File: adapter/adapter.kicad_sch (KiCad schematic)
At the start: 11 parts, among them J1 Serial, J2 Conn_01x05_Female, J3 Conn_01x06_Female, J4 RGB, J7 Trackball, SW1 Reset, U1 STM32F401 / STM32F411 Blackpi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

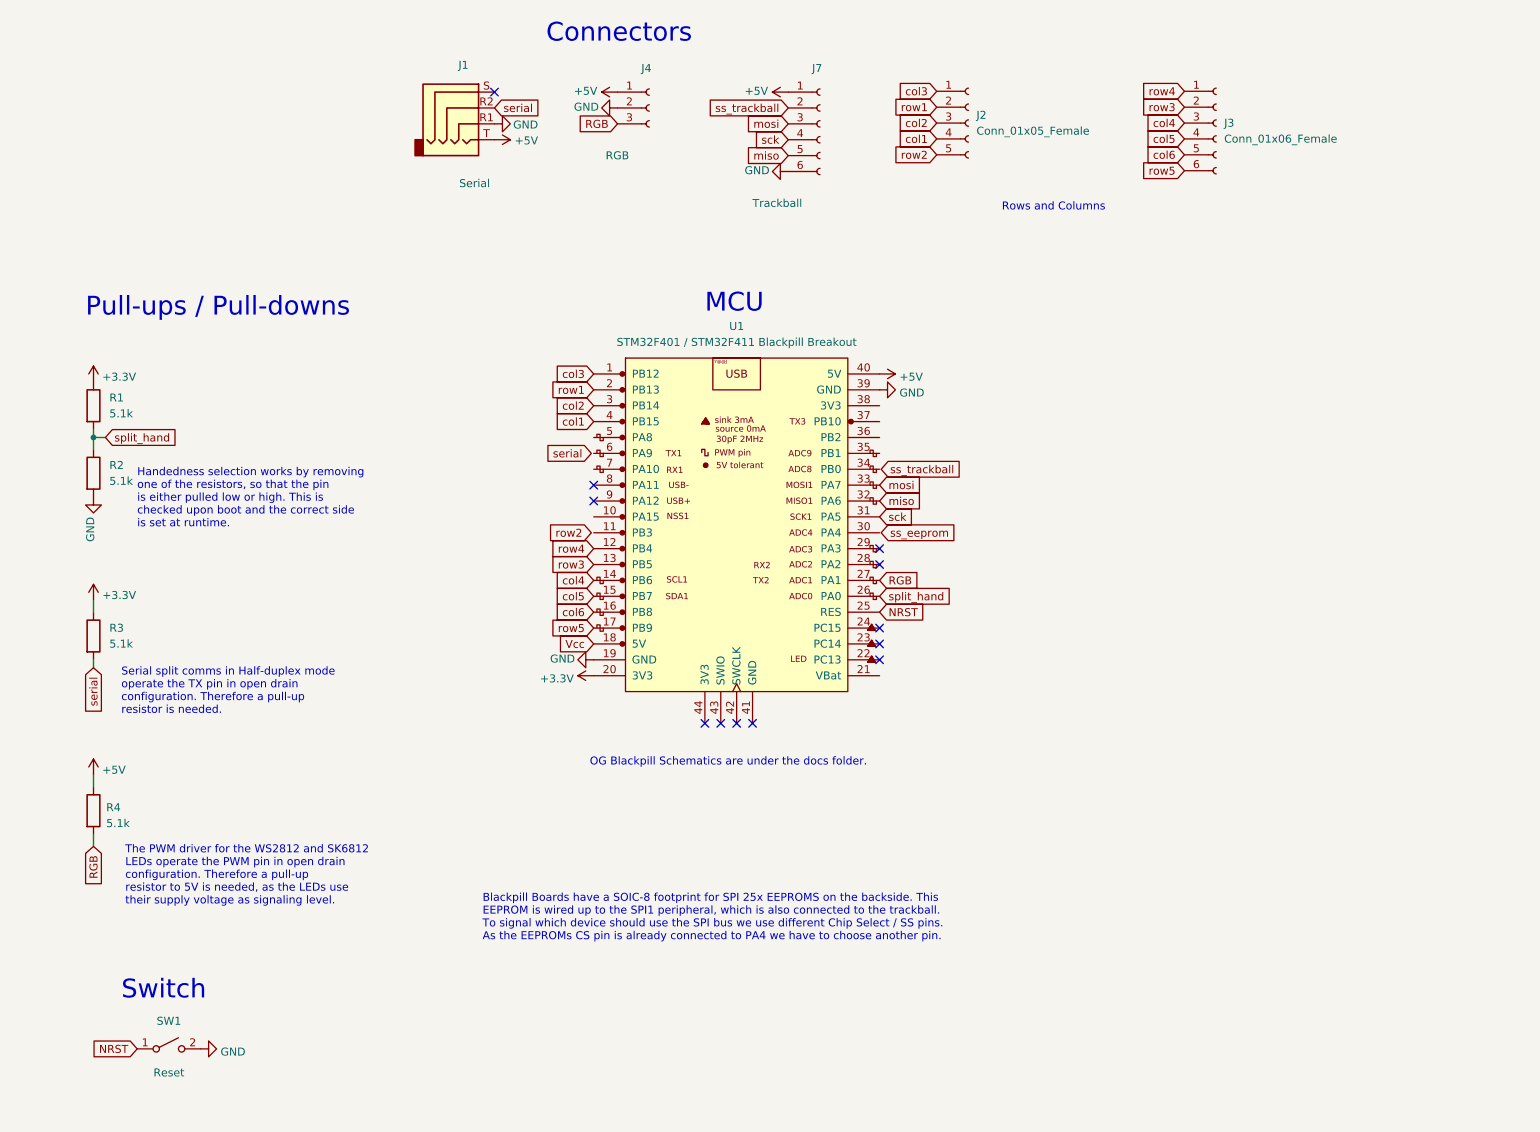
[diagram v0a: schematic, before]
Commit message: Update schematic for left and right hand
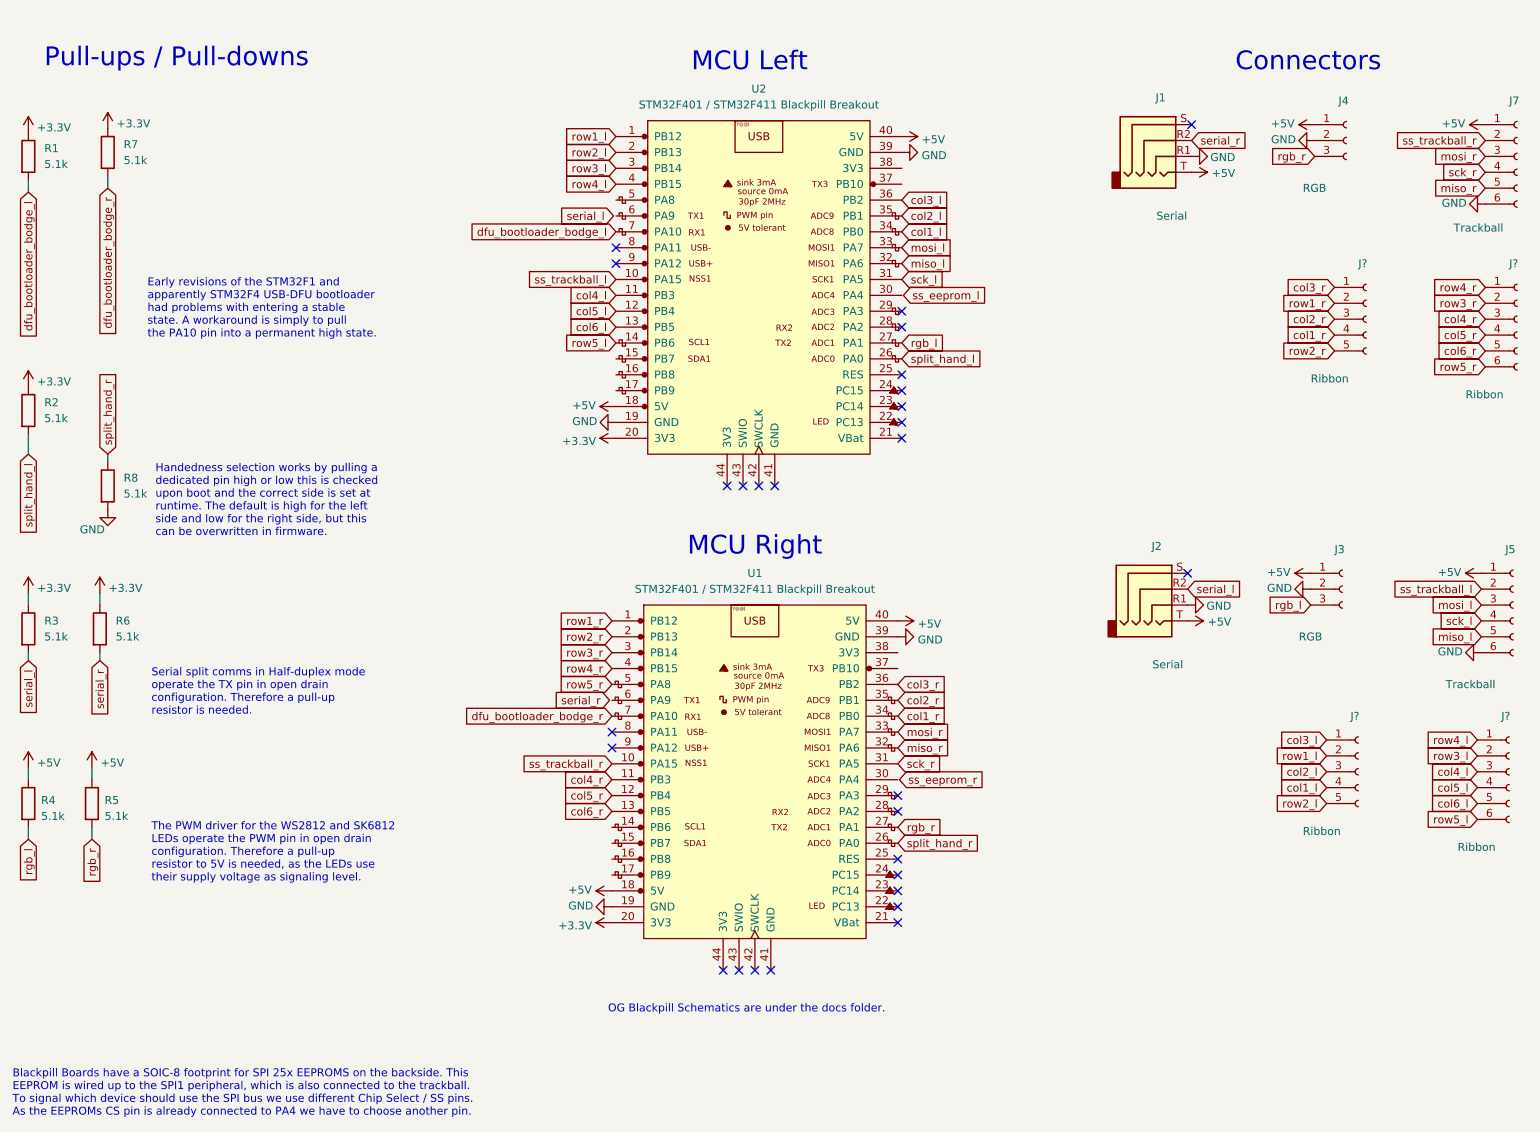
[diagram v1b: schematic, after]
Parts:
- removed J2: Conn_01x05_Female, customs:PinHeader_1x05_P2.54mm_Vertical, symbol Connector:Conn_01x05_Female
- removed J3: Conn_01x06_Female, Connector_PinHeader_2.54mm:PinHeader_1x06_P2.54mm_Vertical, symbol Connector:Conn_01x06_Female
- removed SW1: Reset, customs:switch_rst, symbol Switch:SW_SPST
- added J2: Serial, Library:Jack_3.5mm_PJ320E_Horizontal, symbol Connector:AudioJack4
- added J3: RGB, Connector_PinSocket_2.54mm:PinSocket_1x03_P2.54mm_Vertical, symbol Connector:Conn_01x03_Female
- added J5: Trackball, Connector_PinHeader_2.54mm:PinHeader_1x06_P2.54mm_Vertical, symbol Connector:Conn_01x06_Female
- added J? (x2): Ribbon, customs:PinHeader_1x05_P2.54mm_Vertical, symbol Connector:Conn_01x05_Female
- added J? (x2): Ribbon, Connector_PinHeader_2.54mm:PinHeader_1x06_P2.54mm_Vertical, symbol Connector:Conn_01x06_Female
- added R1, R5, R6, R7: 5.1k, Resistor_SMD:R_0805_2012Metric_Pad1.20x1.40mm_HandSolder, symbol Device:R
- added U1: STM32F401 / STM32F411 Blackpill Breakout, Library:YAAJ_WeAct_BlackPill_SWD_2, symbol YAAJ_WeAct_BlackPill_Part_Like_SWD_Breakout:YAAJ_WeAct_BlackPill_Part_Like_SWD_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
- J1, J4, J7: JLCPCB BOM (none) -> 0
- R2: renamed from R1; footprint (none) -> Resistor_SMD:R_0805_2012Metric_Pad1.20x1.40mm_HandSolder; JLCPCB BOM (none) -> 1; JLCPCB Part (none) -> C27834
- R3, R4: footprint (none) -> Resistor_SMD:R_0805_2012Metric_Pad1.20x1.40mm_HandSolder; JLCPCB BOM (none) -> 1; JLCPCB Part (none) -> C27834
- R8: renamed from R2; footprint (none) -> Resistor_SMD:R_0805_2012Metric_Pad1.20x1.40mm_HandSolder; JLCPCB BOM (none) -> 1; JLCPCB Part (none) -> C27834
- U2: renamed from U1; JLCPCB BOM (none) -> 0
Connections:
- net Vcc is gone; now on net +5V: U2.18 (5V)
- net +3V3: now also R1.1, R6.1, R7.1, U1.20 (3V3)
- net +5V: now also J2.T, J3.1 (Pin_1), J5.1 (Pin_1), R5.1, U1.18 (5V), U1.40 (5V)
- net GND: now also J2.R1, J3.2 (Pin_2), J5.6 (Pin_6), U1.19 (GND), U1.39 (GND)
- net ss_trackball_l: now reaches U2.10 (PA15)
- net ss_trackball_l: now also J5.2 (Pin_2)
- net col4_l: now reaches U2.11 (PB3)
- net col4_l: now also J?.3 (Pin_3)
- net col1_l: now reaches U2.34 (PB0)
- net col1_l: now also J?.4 (Pin_4)
- net col2_l: now reaches U2.35 (PB1)
- net col2_l: now also J?.3 (Pin_3)
- net col3_l: now reaches U2.36 (PB2)
- net col3_l: now also J?.1 (Pin_1)
- net dfu_bootloader_bodge_l: now reaches U2.7 (PA10)
- net dfu_bootloader_bodge_l: now also R1.2
- net NRST: no longer names the net of U2.25 (RES)
- net RGB renamed rgb_l
- net rgb_l: now also J3.3 (Pin_3); no longer J4.3 (Pin_3)
- net col1 renamed row4_l
- net row4_l: now also J?.1 (Pin_1)
- net col2 renamed row3_l
- net row3_l: now also J?.2 (Pin_2)
- net col3 renamed row1_l
- net row1_l: now also J?.2 (Pin_2)
- net col4 renamed row5_l
- net row5_l: now also J?.6 (Pin_6)
- net col5: no longer names the net of U2.15 (PB7)
- net col6: no longer names the net of U2.16 (PB8)
- net miso renamed miso_l
- net miso_l: now also J5.5 (Pin_5); no longer J7.5 (Pin_5)
- net mosi renamed mosi_l
- net mosi_l: now also J5.3 (Pin_3); no longer J7.3 (Pin_3)
- net row1 renamed row2_l
- net row2_l: now also J?.5 (Pin_5)
- net row3 renamed col6_l
- net col6_l: now also J?.5 (Pin_5)
- net row4 renamed col5_l
- net col5_l: now also J?.4 (Pin_4)
- net row5: no longer names the net of U2.17 (PB9)
- net sck renamed sck_l
- net sck_l: now also J5.4 (Pin_4); no longer J7.4 (Pin_4)
- net serial renamed serial_l
- net serial_l: now also J2.R2; no longer J1.R2
- net split_hand renamed split_hand_l
- net split_hand_l: no longer R8.1
- net ss_trackball renamed ss_trackball_r
- net ss_trackball_r: now also U1.10 (PA15)
- new net col1_r: J?.4 (Pin_4), U1.34 (PB0)
- new net col2_r: J?.3 (Pin_3), U1.35 (PB1)
- new net col3_r: J?.1 (Pin_1), U1.36 (PB2)
- new net col4_r: J?.3 (Pin_3), U1.11 (PB3)
- new net col5_r: J?.4 (Pin_4), U1.12 (PB4)
- new net col6_r: J?.5 (Pin_5), U1.13 (PB5)
- new net dfu_bootloader_bodge_r: R7.2, U1.7 (PA10)
- new net miso_r: J7.5 (Pin_5), U1.32 (PA6)
- new net mosi_r: J7.3 (Pin_3), U1.33 (PA7)
- new net rgb_r: J4.3 (Pin_3), R5.2, U1.27 (PA1)
- new net row1_r: J?.2 (Pin_2), U1.1 (PB12)
- new net row2_r: J?.5 (Pin_5), U1.2 (PB13)
- new net row3_r: J?.2 (Pin_2), U1.3 (PB14)
- new net row4_r: J?.1 (Pin_1), U1.4 (PB15)
- new net row5_r: J?.6 (Pin_6), U1.5 (PA8)
- new net sck_r: J7.4 (Pin_4), U1.31 (PA5)
- new net serial_r: J1.R2, R6.2
- new net split_hand_r: R8.1, U1.26 (PA0)
- no-connect marks 12 -> 28
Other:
- note added: "Early revisions of the STM32F1 and apparently STM32F4 USB-DFU bootloader had problems with entering a stable state. A workaround is simply to pull the PA10 pin into a permanent high state."
- note added: "Handedness selection works by pulling a dedicated pin high or low this is checked upon boot and the correct side is set at runtime. The default is high for the left side and low for the right side, but this can be overwritten in firmware."
- note added: "MCU Left"
- note added: "MCU Right"
- note removed: "Handedness selection works by removing one of the resistors, so that the pin is either pulled low or high. This is checked upon boot and the correct side is set at runtime."
- note removed: "MCU"
- note removed: "Rows and Columns"
- note removed: "Switch"
- company: (none) -> Bastardkb x KarlK90
- title: (none) -> Charybdis Blackpill Holder
- moved on the sheet: J1, J4, J7, R2, R3, R4, R8, U2

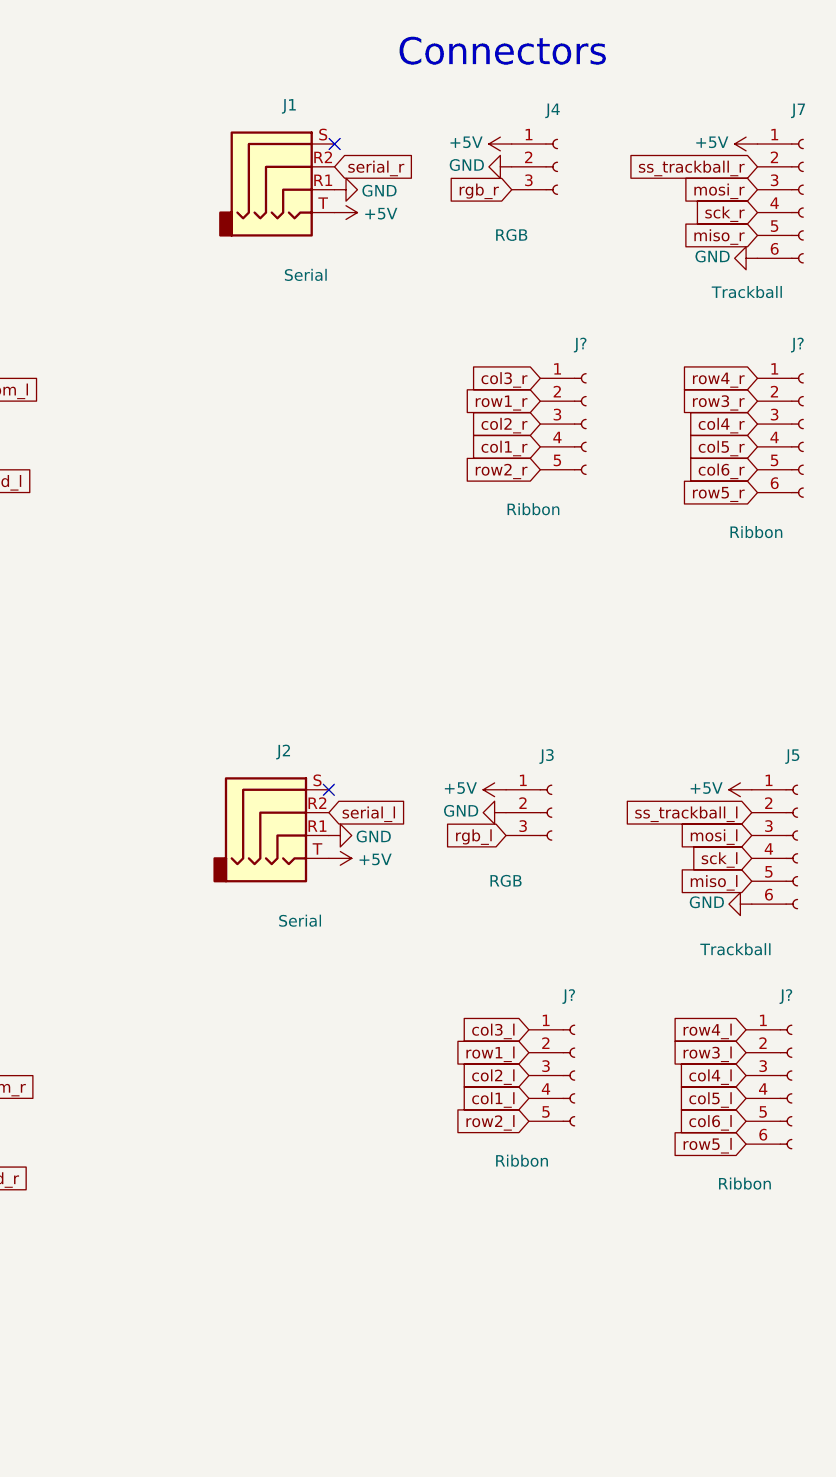
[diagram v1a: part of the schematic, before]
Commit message: fix connection placement
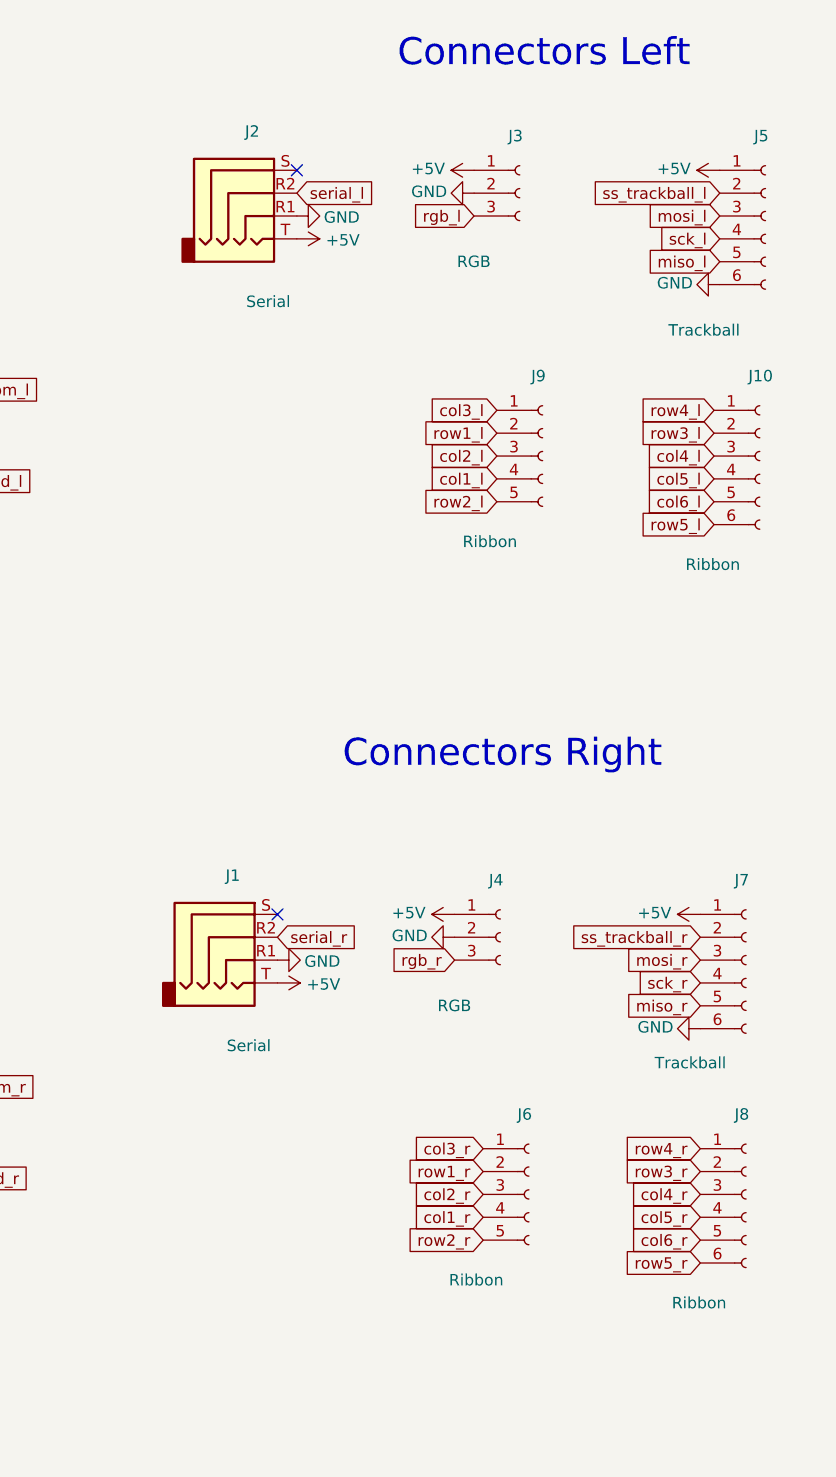
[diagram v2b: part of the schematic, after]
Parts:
- gave numbers to parts that had none: 4
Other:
- note added: "Connectors Left"
- note added: "Connectors Right"
- note removed: "Connectors"
- moved on the sheet: J1, J10, J2, J3, J4, J5, J6, J7, J8, J9

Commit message: component placement
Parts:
- J6: footprint customs:PinHeader_1x05_P2.54mm_Vertical -> Connector_PinHeader_2.54mm:PinHeader_1x05_P2.54mm_Vertical
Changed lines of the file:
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@@
       (effects (font (size 1.27 1.27)) (justify left))
     )
-    (property "Footprint" "customs:PinHeader_1x05_P2.54mm_Vertical" (id 2) (at 231.775 149.733 0)
+    (property "Footprint" "Connector_PinHeader_2.54mm:PinHeader_1x05_P2.54mm_Vertical" (id 2) (at 231.775 149.733 0)
       (effects (font (size 1.27 1.27)) hide)
     )
@@
     )
     (path "/45f0799c-408b-4e0d-8bc6-8ee6ccaf8219"
-      (reference "J6") (unit 1) (value "Ribbon") (footprint "customs:PinHeader_1x05_P2.54mm_Vertical")
+      (reference "J6") (unit 1) (value "Ribbon") (footprint "Connector_PinHeader_2.54mm:PinHeader_1x05_P2.54mm_Vertical")
     )
     (path "/7bffcea9-b23e-4698-8571-09d538a5c739"
